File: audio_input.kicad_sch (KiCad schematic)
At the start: 64 parts, among them J11 NCJ6FA-H-0, J12 NCJ6FA-H-0, Q2 2N3904, Q3 2N3904, Q4 2N3906, Q5 2N3906, U10 THAT1246, U7 OPA1656ID, U8 LM2903, U9 THAT1246

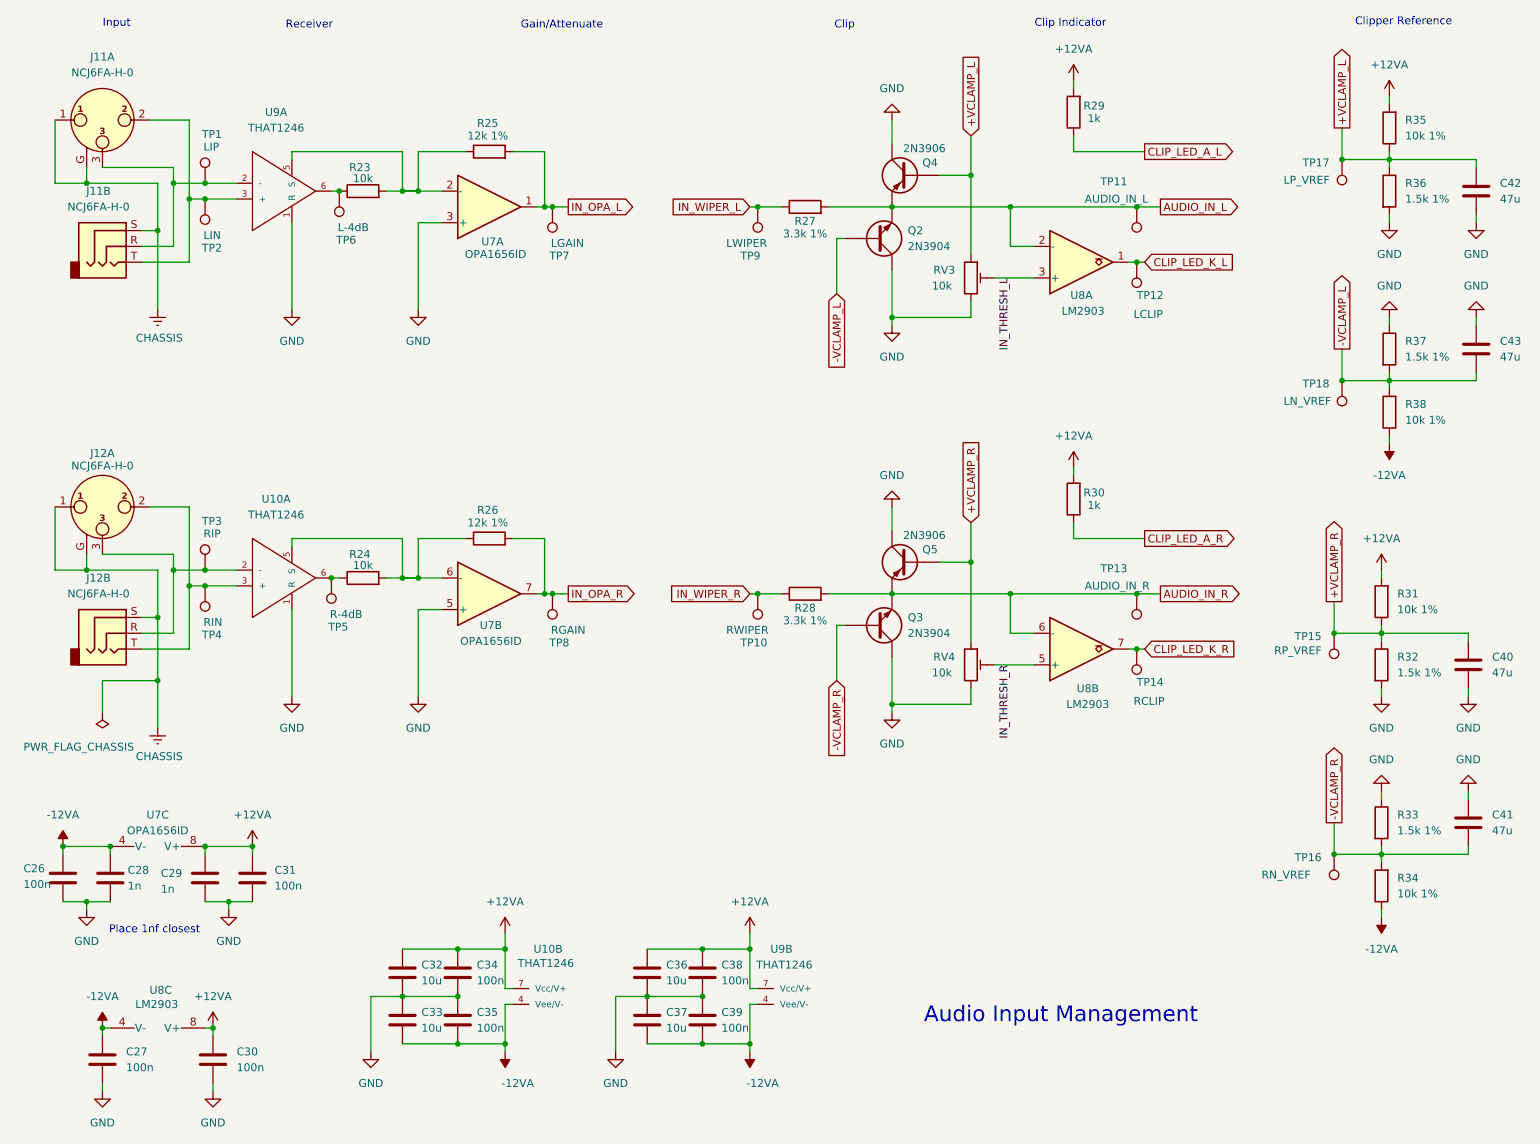
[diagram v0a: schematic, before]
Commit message: lots of pcb work
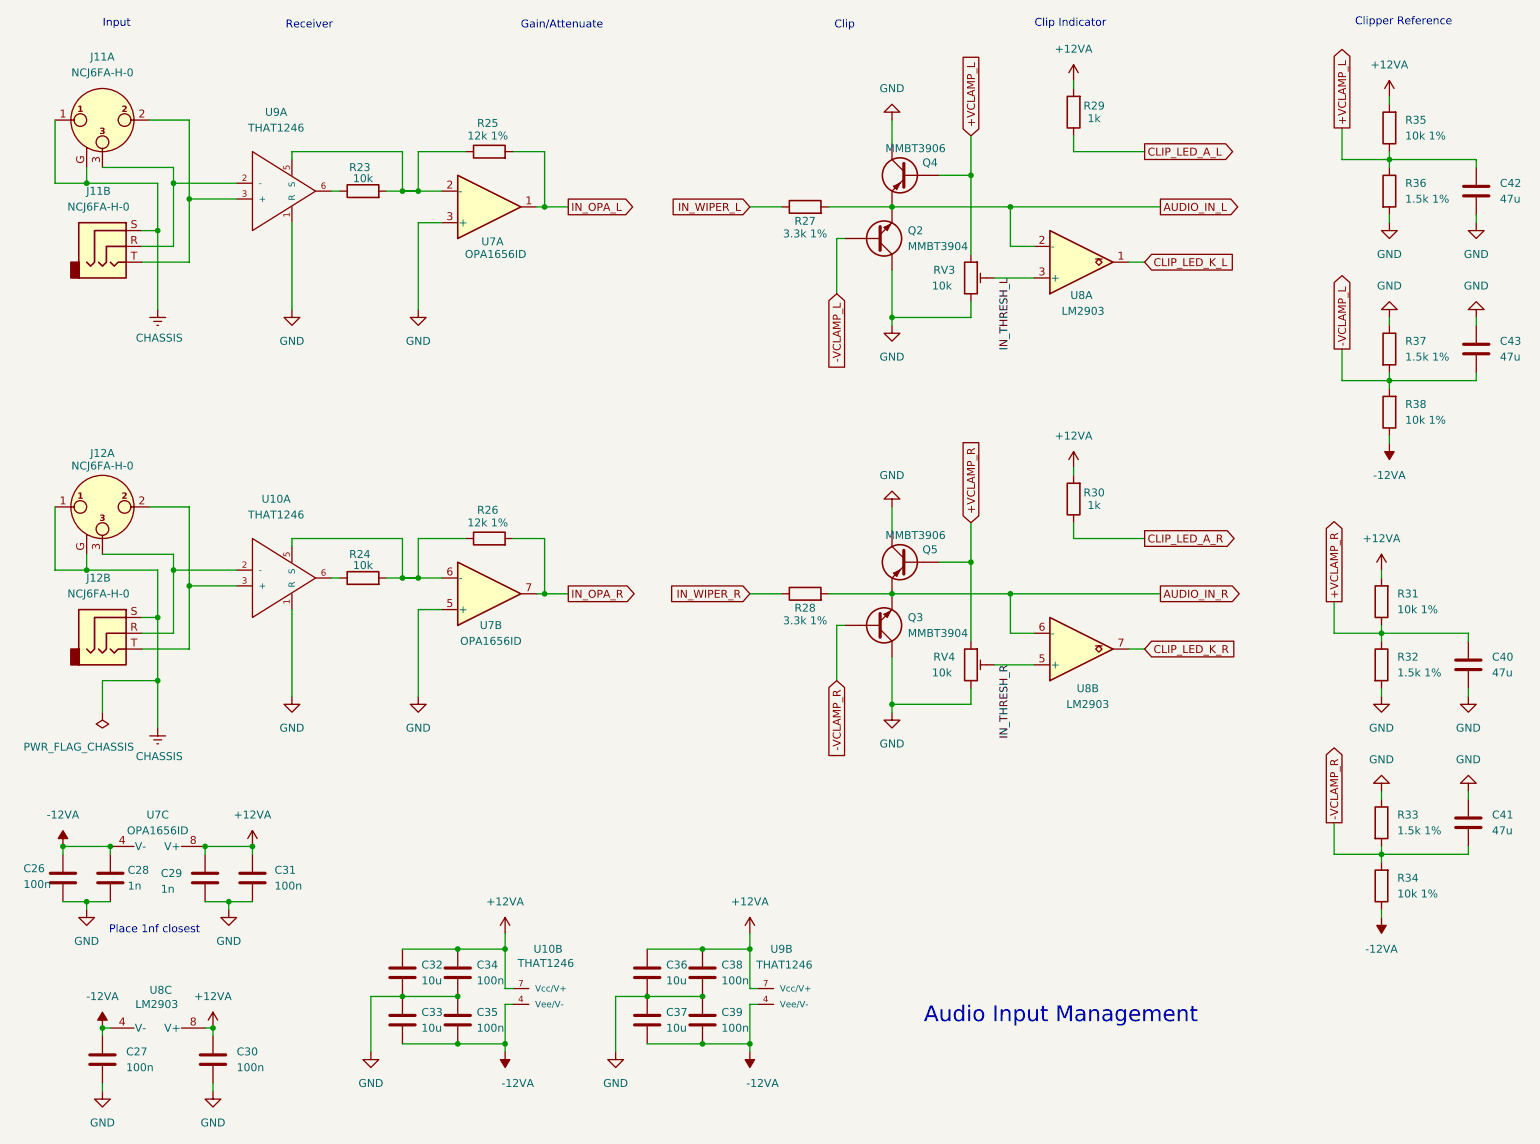
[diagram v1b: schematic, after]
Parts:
- removed TP1: LIP, TestPoint:TestPoint_Pad_1.5x1.5mm, symbol Connector:TestPoint
- removed TP10: RWIPER, TestPoint:TestPoint_Pad_1.5x1.5mm, symbol Connector:TestPoint
- removed TP11: AUDIO_IN_L, TestPoint:TestPoint_Pad_1.5x1.5mm, symbol Connector:TestPoint
- removed TP12: LCLIP, TestPoint:TestPoint_Pad_1.5x1.5mm, symbol Connector:TestPoint
- removed TP13: AUDIO_IN_R, TestPoint:TestPoint_Pad_1.5x1.5mm, symbol Connector:TestPoint
- removed TP14: RCLIP, TestPoint:TestPoint_Pad_1.5x1.5mm, symbol Connector:TestPoint
- removed TP15: RP_VREF, TestPoint:TestPoint_Pad_1.5x1.5mm, symbol Connector:TestPoint
- removed TP16: RN_VREF, TestPoint:TestPoint_Pad_1.5x1.5mm, symbol Connector:TestPoint
- removed TP17: LP_VREF, TestPoint:TestPoint_Pad_1.5x1.5mm, symbol Connector:TestPoint
- removed TP18: LN_VREF, TestPoint:TestPoint_Pad_1.5x1.5mm, symbol Connector:TestPoint
- removed TP2: LIN, TestPoint:TestPoint_Pad_1.5x1.5mm, symbol Connector:TestPoint
- removed TP3: RIP, TestPoint:TestPoint_Pad_1.5x1.5mm, symbol Connector:TestPoint
- removed TP4: RIN, TestPoint:TestPoint_Pad_1.5x1.5mm, symbol Connector:TestPoint
- removed TP5: R-4dB, TestPoint:TestPoint_Pad_1.5x1.5mm, symbol Connector:TestPoint
- removed TP6: L-4dB, TestPoint:TestPoint_Pad_1.5x1.5mm, symbol Connector:TestPoint
- removed TP7: LGAIN, TestPoint:TestPoint_Pad_1.5x1.5mm, symbol Connector:TestPoint
- removed TP8: RGAIN, TestPoint:TestPoint_Pad_1.5x1.5mm, symbol Connector:TestPoint
- removed TP9: LWIPER, TestPoint:TestPoint_Pad_1.5x1.5mm, symbol Connector:TestPoint
- Q2, Q3: value 2N3904 -> MMBT3904; footprint Package_TO_SOT_THT:TO-92_Inline -> Package_TO_SOT_SMD:SOT-23
- Q4, Q5: value 2N3906 -> MMBT3906; footprint Package_TO_SOT_THT:TO-92_Inline -> Package_TO_SOT_SMD:SOT-23

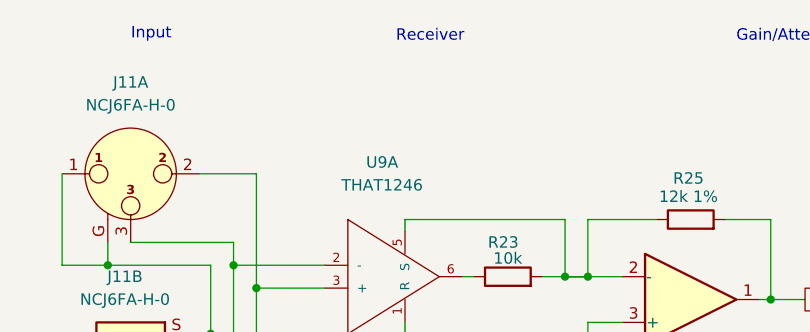
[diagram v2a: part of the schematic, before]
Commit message: lots of pcb work
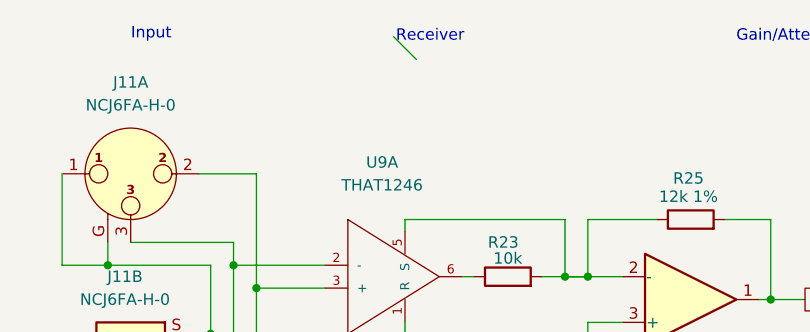
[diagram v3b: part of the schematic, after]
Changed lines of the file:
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@@
 		(color 0 0 0 0)
+	)
+	(bus_entry
+		(at 60.96 17.78)
+		(size 2.54 2.54)
+		(stroke
+			(width 0)
+			(type default)
+		)
 	)
 	(wire
